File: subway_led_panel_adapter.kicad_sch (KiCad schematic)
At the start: 59 parts

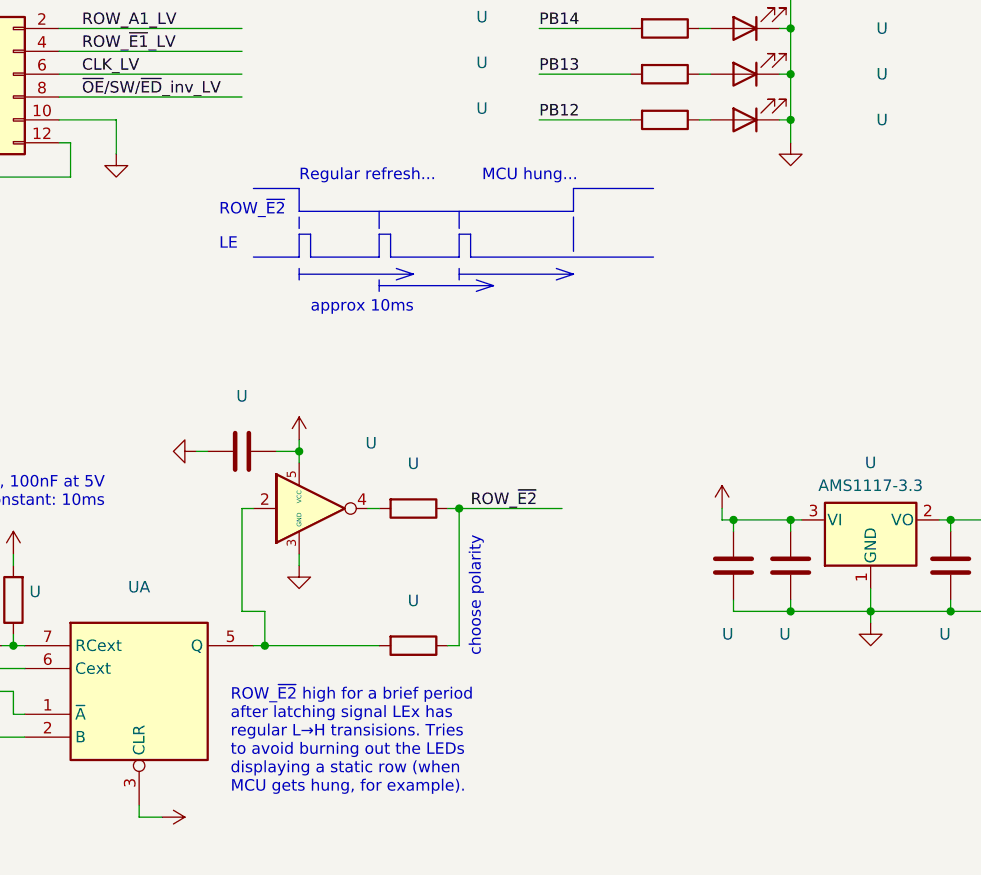
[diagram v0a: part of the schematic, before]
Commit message: Cleanup rev. B.
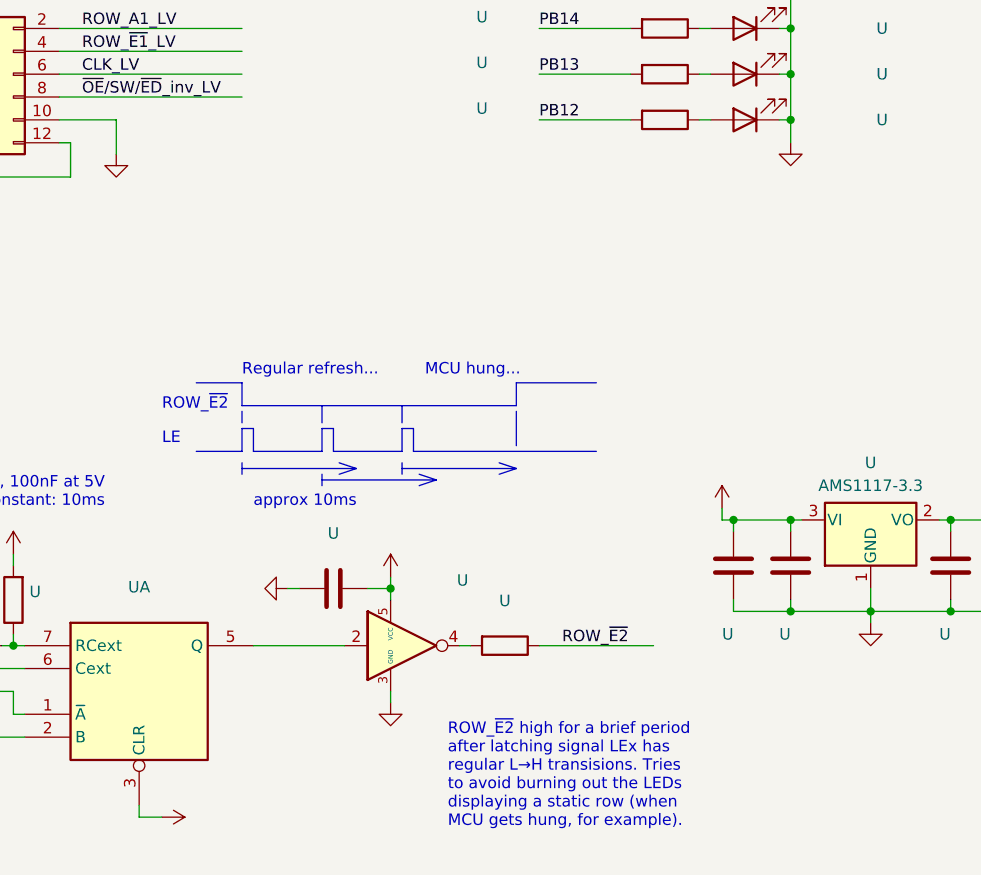
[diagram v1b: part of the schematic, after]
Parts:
- removed U: (no value), symbol Device:R
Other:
- note removed: "choose polarity"
- moved on the sheet: U
